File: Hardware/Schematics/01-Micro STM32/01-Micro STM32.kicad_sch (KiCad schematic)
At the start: 51 parts, among them J1 Conn_01x06, J10 USB_B_Mini, J2 Conn_02x05_Odd_Even, J3 Conn_02x25_Odd_Even, J4 Conn_01x04, J5 Conn_01x12, J6 Micro_SD_Card_Det1, J9 USB_B, Q1 BC817, SW1 SW_DIP_x05, U1 MCP23017_ML, U10 BQ25172DSGR, U11 LDL112-LD0, U2 ESP32-DEVKITC-32D, U3 74HCT138, U4 74HCT138, U5 CP2102N-Axx-xQFN28, U6 USBLC6-2SC6, U69A AD8604ARUZ, U7 74HC04, U8 LM1117MP-3.3

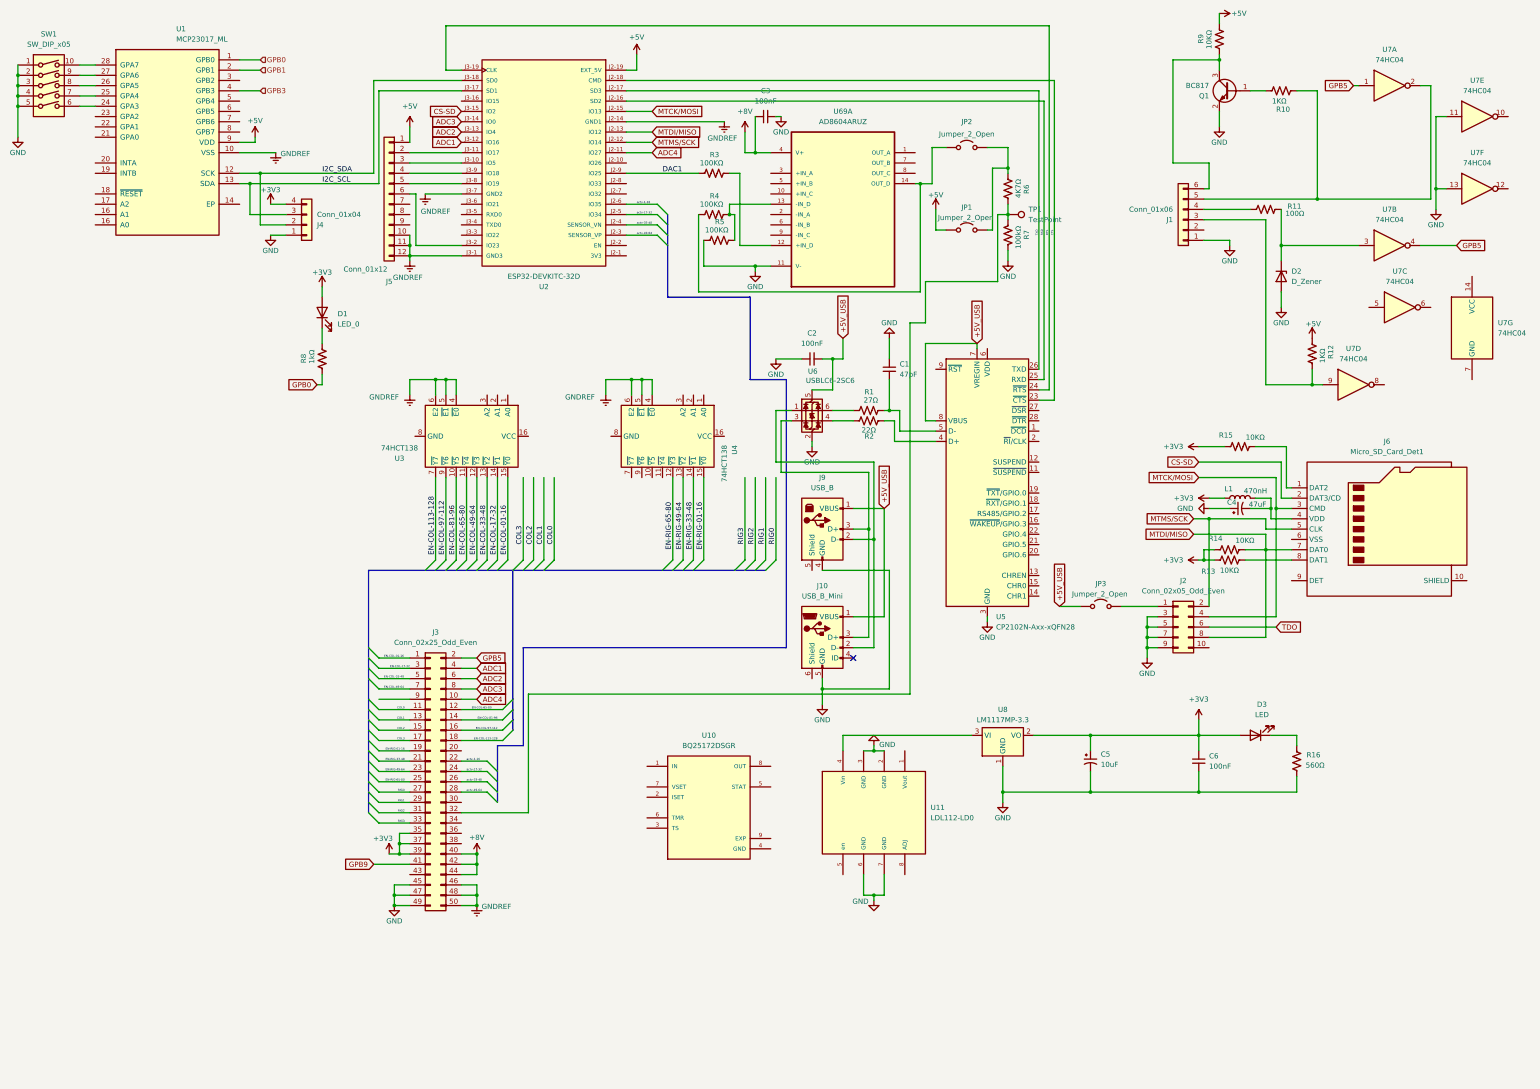
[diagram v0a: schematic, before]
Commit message: Finalized Schematic
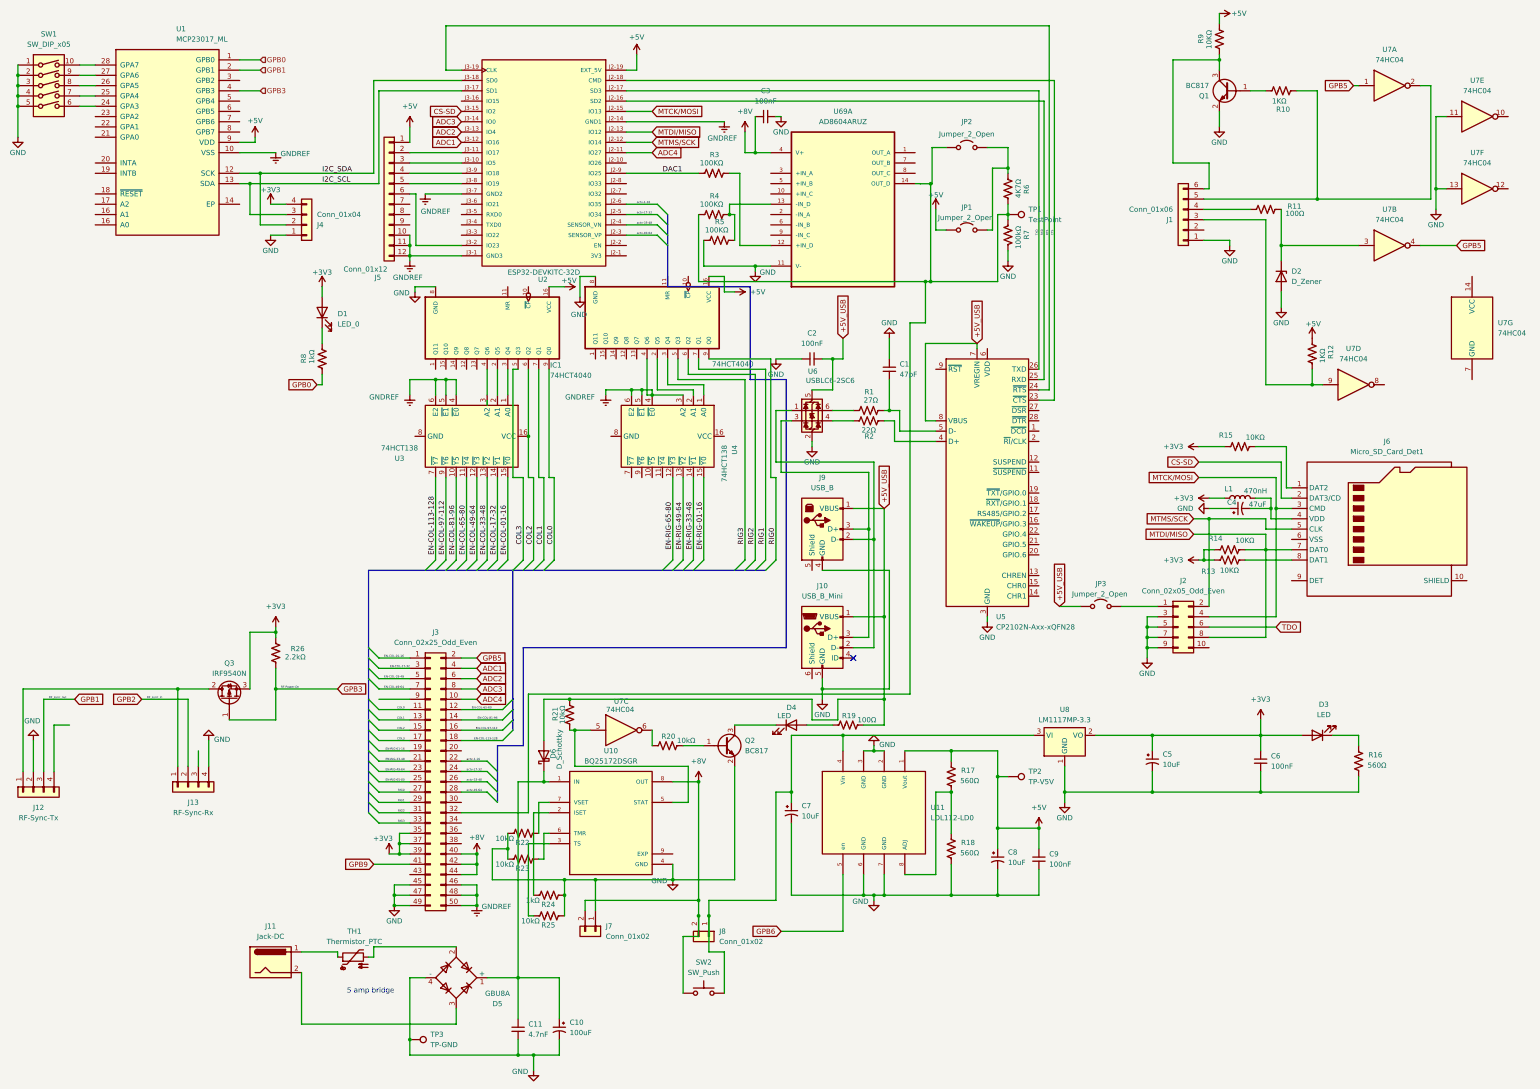
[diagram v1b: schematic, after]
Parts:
- added C10: 100uF, symbol Device:C_Polarized_Small_US
- added C11: 4.7nF, symbol Device:C_Small
- added C7, C8: 10uF, symbol Device:C_Polarized_Small_US
- added C9: 100nF, symbol Device:C_Small
- added D4: LED, symbol Device:LED
- added D5: GBU8A, Diode_THT:Diode_Bridge_Vishay_GBU, symbol Diode_Bridge:GBU8A
- added D6: D_Schottky, symbol Device:D_Schottky
- added IC1, IC2: 74HCT4040, 74HCT4040:TSSOP16, symbol 74HCT4040:74HCT4040
- added J11: Jack-DC, symbol Connector:Jack-DC
- added J12: RF-Sync-Tx, symbol Connector_Generic:Conn_01x04
- added J13: RF-Sync-Rx, symbol Connector_Generic:Conn_01x04
- added J7, J8: Conn_01x02, symbol Connector_Generic:Conn_01x02
- added Q2: BC817, Package_TO_SOT_SMD:SOT-23, symbol Transistor_BJT:BC817
- added Q3: IRF9540N, Package_TO_SOT_THT:TO-220-3_Vertical, symbol Transistor_FET:IRF9540N
- added R17, R18: 560Ω, symbol Device:R_US
- added R19: 100Ω, symbol Device:R_US
- added R20, R21, R22, R23, R25: 10kΩ, symbol Device:R_US
- added R24: 1kΩ, symbol Device:R_US
- added R26: 2.2kΩ, symbol Device:R_US
- added SW2: SW_Push, symbol Switch:SW_Push
- added TH1: Thermistor_PTC, symbol Device:Thermistor_PTC
- added TP2: TP-V5V, symbol Connector:TestPoint
- added TP3: TP-GND, symbol Connector:TestPoint
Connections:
- net +3V3: now also Q3.3 (S), R26.2
- net +5V: now also U11.1 (Vout), C8.1, C9.1, IC1.16 (VCC), IC2.16 (VCC), R17.2, TP2.1
- net +5V_USB: now also D6.2 (A), R19.1, R21.1
- net +8V: now also U10.8 (OUT), J7.2 (Pin_2), J8.2 (Pin_2), SW2.1
- net COL0: now also IC1.9 (Q0)
- net COL1: now also IC1.7 (Q1)
- net COL2: now also U3.16 (VCC), IC1.6 (Q2)
- net COL3: now also IC1.5 (Q3)
- net GND: now also U10.4 (GND), C10.2, C11.2, C7.2, C8.2, C9.2, D5.4 (-), IC1.8 (GND), IC2.8 (GND), J12.2 (Pin_2), J13.4 (Pin_4), J7.1 (Pin_1), Q2.2 (E), R18.1, R22.1, R23.1, R24.2, R25.2, TP3.1
- net GNDREF: now also U4.3 (A2), IC2.4 (Q6)
- net GPB1: now also J12.3 (Pin_3)
- net GPB3: now also Q3.1 (G), R26.1
- net RIG0: now also IC2.9 (Q0)
- net RIG1: now also IC2.7 (Q1)
- net RIG2: now also IC2.6 (Q2)
- net RIG3: now also IC2.5 (Q3)
- net at U11.4 (Vin), U8.3 (VI): now also C7.1, J8.1 (Pin_1), SW2.2
- net GPB6: now reaches U11.5 (en)
- net at U11.8 (ADJ): now also R17.1, R18.2
- net at U4.1 (A0): now also IC2.3 (Q4)
- net at U4.2 (A1): now also IC2.2 (Q5)
- net at JP2.1 (A), R4.1, U69A.14 (OUT_D): now also J3.32 (Pin_32), R6.2, R7.2, TP1.1
- net at U7.5: now also U10.5 (STAT), R21.2
- net at U7.6: now also R20.2
- net at U10.1 (IN): now also C10.1, C11.1, D5.1 (+), D6.1 (K)
- net at U10.2 (ISET): now also R24.1
- net at U10.3 (TS): now also R25.1
- net at U10.6 (TMR): now also R23.2
- net at U10.7 (VSET): now also R22.2
- net at U3.1 (A0): now also IC1.3 (Q4)
- net at U3.2 (A1): now also IC1.2 (Q5)
- net at U3.3 (A2): now also IC1.4 (Q6)
- new net: J12.1 (Pin_1), J13.1 (Pin_1), Q3.2 (D)
- new net: D4.1 (K), Q2.3 (C)
- new net: D4.2 (A), R19.2
- new net: Q2.1 (B), R20.1
- new net: D5.2, TH1.2
- new net: D5.3, J11.2
- new net: J11.1, TH1.1
- new net GPB2: J13.2 (Pin_2)
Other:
- note added: "5 amp bridge"
- moved on the sheet: C5, C6, D3, R16, U10, U8
